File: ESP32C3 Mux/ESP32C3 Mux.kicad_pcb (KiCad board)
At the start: 2 copper layers, 31.2 x 28.9 mm, 9 parts, among them J1 SSW-104-22-F-D-RA, J2 Conn_01x02_Socket, J3 SSW-104-22-F-D-RA, U1 ESP32C3, U8 STLQ015M33R

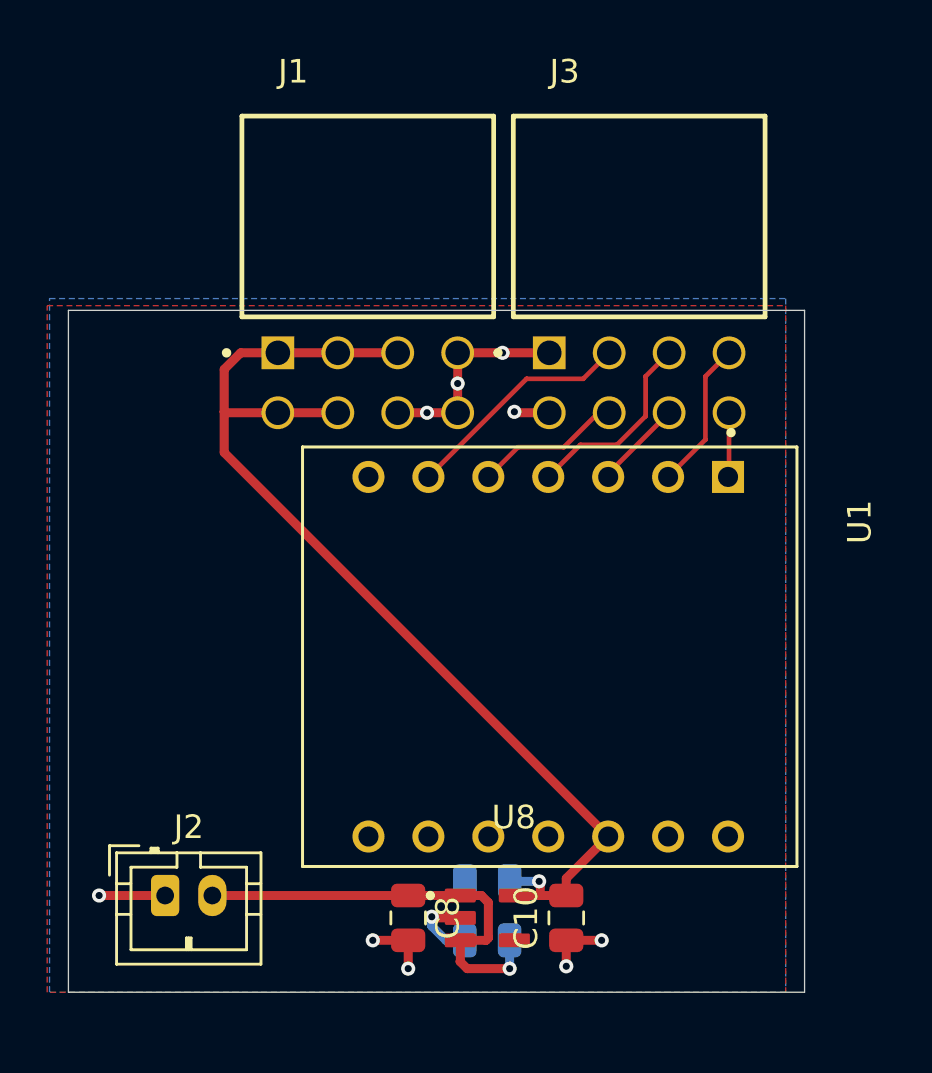
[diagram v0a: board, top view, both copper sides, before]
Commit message: updates
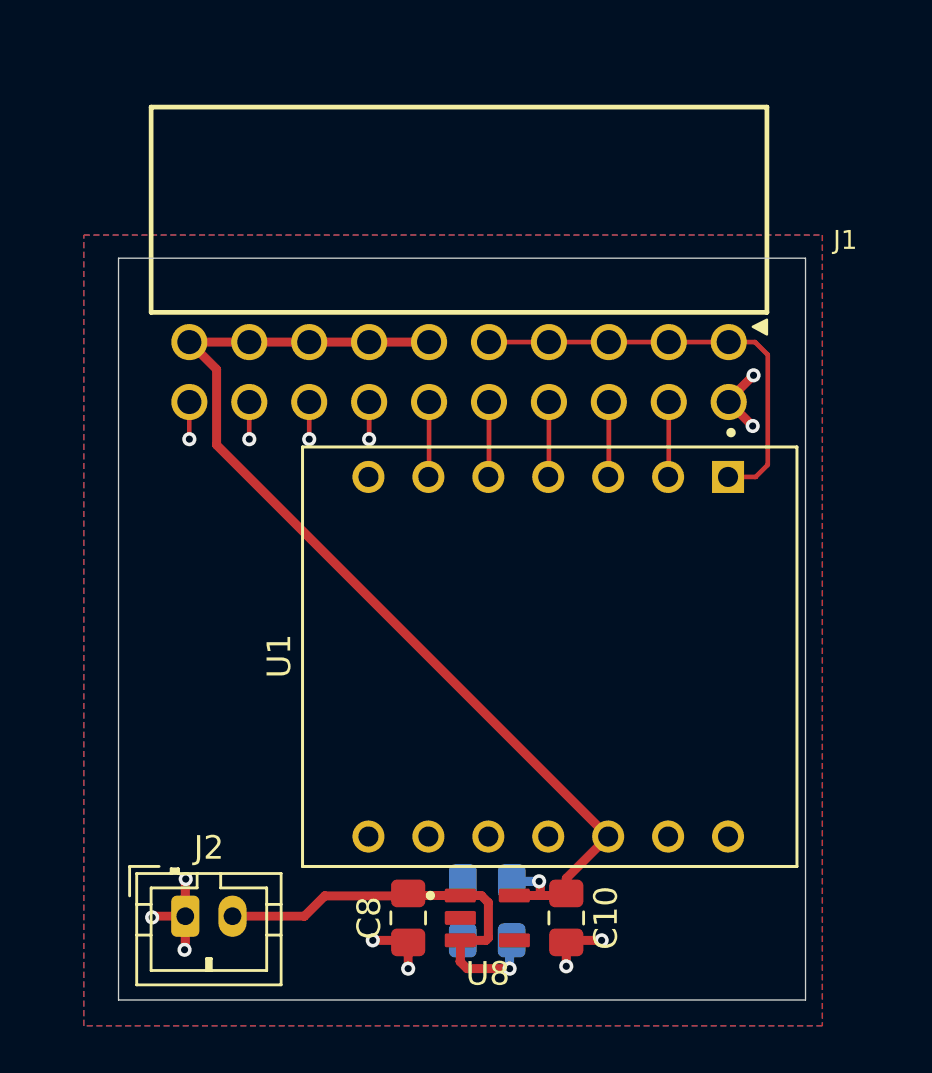
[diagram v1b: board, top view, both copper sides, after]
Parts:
- removed J3: SSW-104-22-F-D-RA, ESP32C3 Mux:SAMTEC_SSW-104-22-F-D-RA
- C10, C7, C8, C9: footprint Capacitor_SMD:C_0805_2012Metric -> Capacitor_SMD:C_0805_2012Metric_Pad1.18x1.45mm_HandSolder
- J1: value SSW-104-22-F-D-RA -> 6130XX243121_613020243121; footprint ESP32C3 Mux:SAMTEC_SSW-104-22-F-D-RA -> ESP32C3 Mux:613020243121
- moved J1 9.78 mm to (162.3, 95.6), turned to 180 degrees
- moved J2 1.22 mm to (150.7, 125.6)
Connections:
- U1 pad 2: /SDA1 -> /SDA0
- U1 pad 3: /SDA2 -> /SDA1
- U1 pad 4: /SDA3 -> /SDA2
- U1 pad 5: /SDA4 -> /SDA3
- U1 pad 6: /SDA5 -> /SDA4
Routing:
- net /SCL: track 2.74 -> 18.6 mm
- net /SDA5: track 9.84 -> 0.00 mm
- net /SDA3: track 8.29 -> 3.19 mm
- net /SDA1: track 6.72 -> 3.19 mm
- net /SDA0: track 0.00 -> 3.19 mm
- net /SDA4: track 6.25 -> 3.19 mm
- net GND: track 21.8 -> 19.0 mm, vias 10 -> 13
- net /SDA2: track 3.79 -> 3.19 mm
- net +3V3: track 46.3 -> 45.8 mm
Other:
- board size 31.2 x 28.9 mm -> 29.1 x 31.4 mm
